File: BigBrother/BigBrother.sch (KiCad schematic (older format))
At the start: 4 parts, among them U1 bno055, U2 BMP388, U3 VHN5019_Breakout

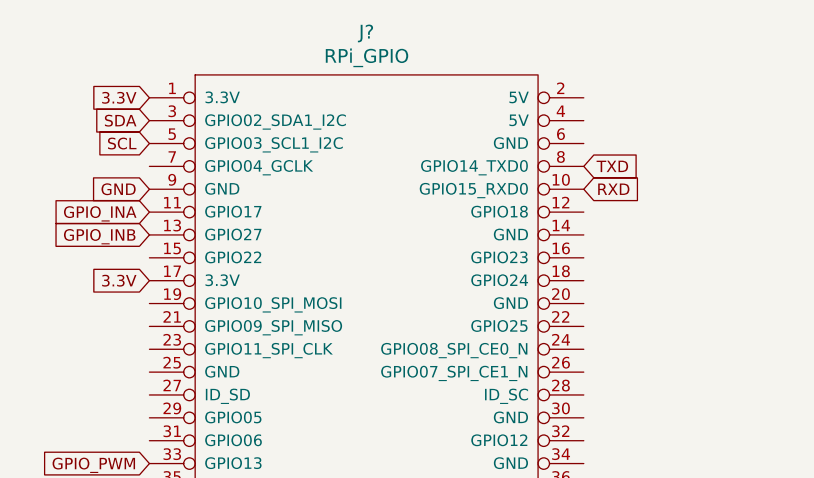
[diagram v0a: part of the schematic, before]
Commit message: Boarddddd
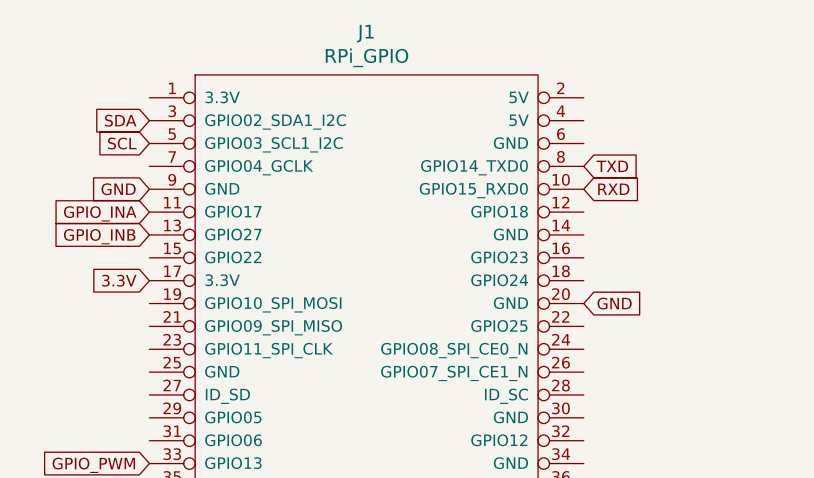
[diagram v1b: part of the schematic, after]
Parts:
- J1: renamed from J?; footprint (none) -> Raspberry Pi Zero:RPI_Zero
- U1: footprint (none) -> NUSTARS:bno055
- U2: footprint MODULE -> BMP388:BMP388
- U3: footprint (none) -> NUSTARS:VNH5019_breakout
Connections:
- net 3.3V: no longer J1.1 (3.3V)
- net GND: now also J1.20 (GND)
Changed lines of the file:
@@
 EESchema Schematic File Version 4
+LIBS:BigBrother-cache
 EELAYER 30 0
 EELAYER END
@@
 $EndDescr
 $Comp
-L Connector-ML:RPi_GPIO J?
-U 1 1 5E488C88
-P 1750 1350
-F 0 "J?" H 2500 1637 60  0000 C CNN
-F 1 "RPi_GPIO" H 2500 1531 60  0000 C CNN
-F 2 "" H 1750 1350 60  0000 C CNN
-F 3 "" H 1750 1350 60  0000 C CNN
-	1    1750 1350
-	1    0    0    -1
-$EndComp
-$Comp
 L BMP388:BMP388 U2
 U 1 1 5E48BA81
@@
 F 0 "U2" H 8778 5046 50  0000 L CNN
 F 1 "BMP388" H 8778 4955 50  0000 L CNN
-F 2 "MODULE" H 8300 5000 50  0001 C CNN
+F 2 "BMP388:BMP388" H 8300 5000 50  0001 C CNN
 F 3 "DOCUMENTATION" H 8300 5000 50  0001 C CNN
 	1    8300 5000
 	1    0    0    -1
 $EndComp
-Text GLabel 1550 1350 0    50   Input ~ 0
-3.3V
 Text GLabel 1550 1750 0    50   Input ~ 0
 GND
@@
 F 0 "U1" H 8300 2265 50  0000 C CNN
 F 1 "bno055" H 8300 2174 50  0000 C CNN
-F 2 "" H 8250 2250 50  0001 C CNN
+F 2 "NUSTARS:bno055" H 8250 2250 50  0001 C CNN
 F 3 "" H 8250 2250 50  0001 C CNN
 	1    7900 2100
@@
 F 0 "U3" H 2475 5275 50  0000 C CNN
 F 1 "VHN5019_Breakout" H 2475 5184 50  0000 C CNN
-F 2 "" H 2900 5200 50  0001 C CNN
+F 2 "NUSTARS:VNH5019_breakout" H 2900 5200 50  0001 C CNN
 F 3 "" H 2900 5200 50  0001 C CNN
 	1    2100 5100
@@
 Text GLabel 2000 5750 0    50   Input ~ 0
 3.3V
+$Comp
+L Connector-ML:RPi_GPIO J1
+U 1 1 5E488C88
+P 1750 1350
+F 0 "J1" H 2500 1637 60  0000 C CNN
+F 1 "RPi_GPIO" H 2500 1531 60  0000 C CNN
+F 2 "Raspberry Pi Zero:RPI_Zero" H 1750 1350 60  0001 C CNN
+F 3 "" H 1750 1350 60  0000 C CNN
+	1    1750 1350
+	1    0    0    -1
+$EndComp
+Text GLabel 3450 2250 2    50   Input ~ 0
+GND
 $EndSCHEMATC

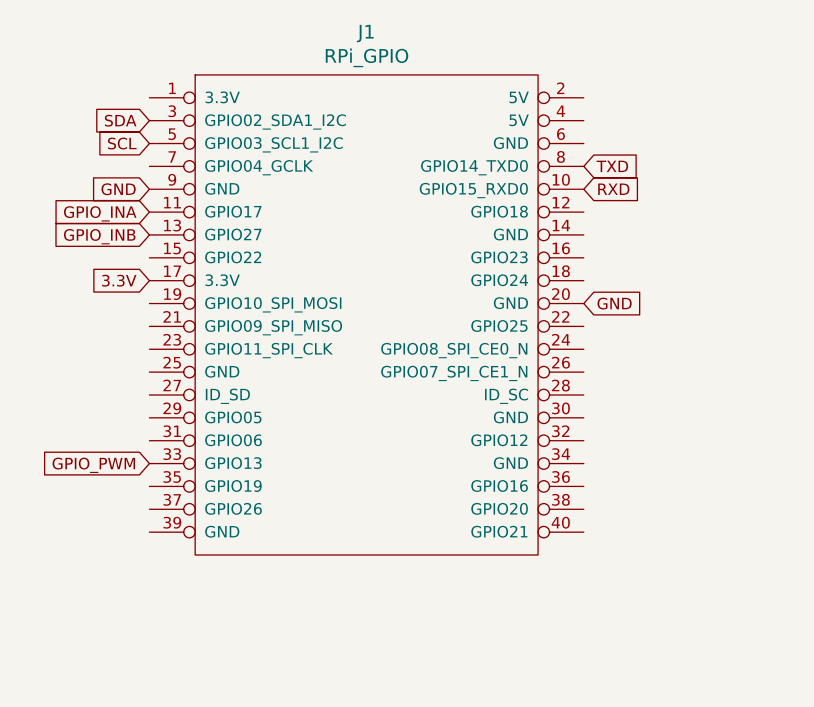
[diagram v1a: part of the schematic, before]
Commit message: Board!! maybe done!!!
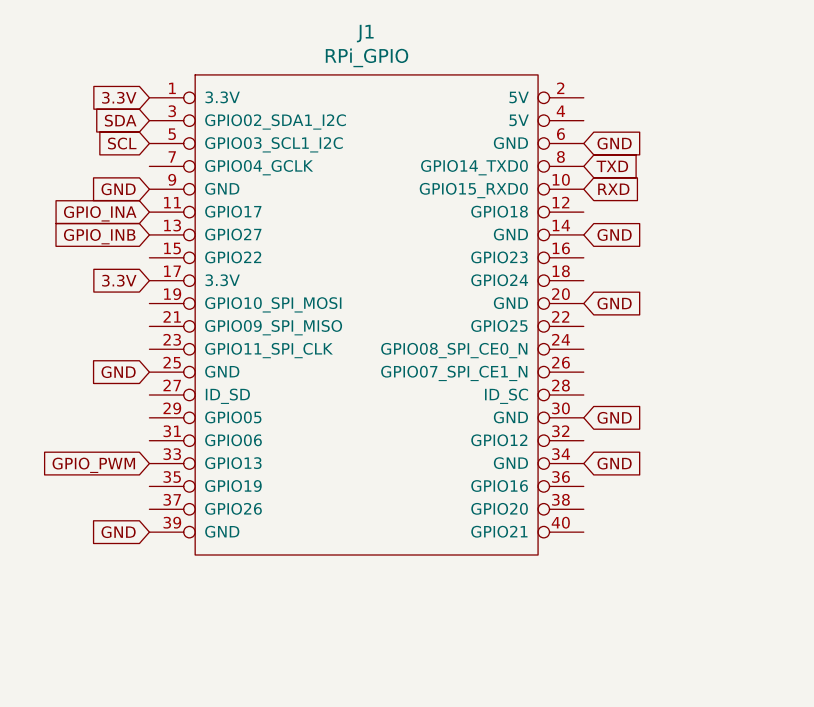
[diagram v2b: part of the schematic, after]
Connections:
- net 3.3V: now also J1.1 (3.3V)
- net GND: now also J1.14 (GND), J1.25 (GND), J1.30 (GND), J1.34 (GND), J1.39 (GND), J1.6 (GND)
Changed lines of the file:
@@
 Text GLabel 3450 2250 2    50   Input ~ 0
 GND
+Text GLabel 1550 1350 0    50   Input ~ 0
+3.3V
+Text GLabel 1550 2550 0    50   Input ~ 0
+GND
+Text GLabel 1550 3250 0    50   Input ~ 0
+GND
+Text GLabel 3450 1550 2    50   Input ~ 0
+GND
+Text GLabel 3450 1950 2    50   Input ~ 0
+GND
+Text GLabel 3450 2750 2    50   Input ~ 0
+GND
+Text GLabel 3450 2950 2    50   Input ~ 0
+GND
 $EndSCHEMATC
